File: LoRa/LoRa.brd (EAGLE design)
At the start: 51.7 x 22.8 mm, 27 parts, among them J1 UP2-AH-1-TH, U1 STM32L053C8T6, U2 RFM69HCW, U3 BSS138, U4 BSS138, U5 LM3671MF-3.3/NOPB, X1 uFL/SMA, Y1 ECS-80-S-4X

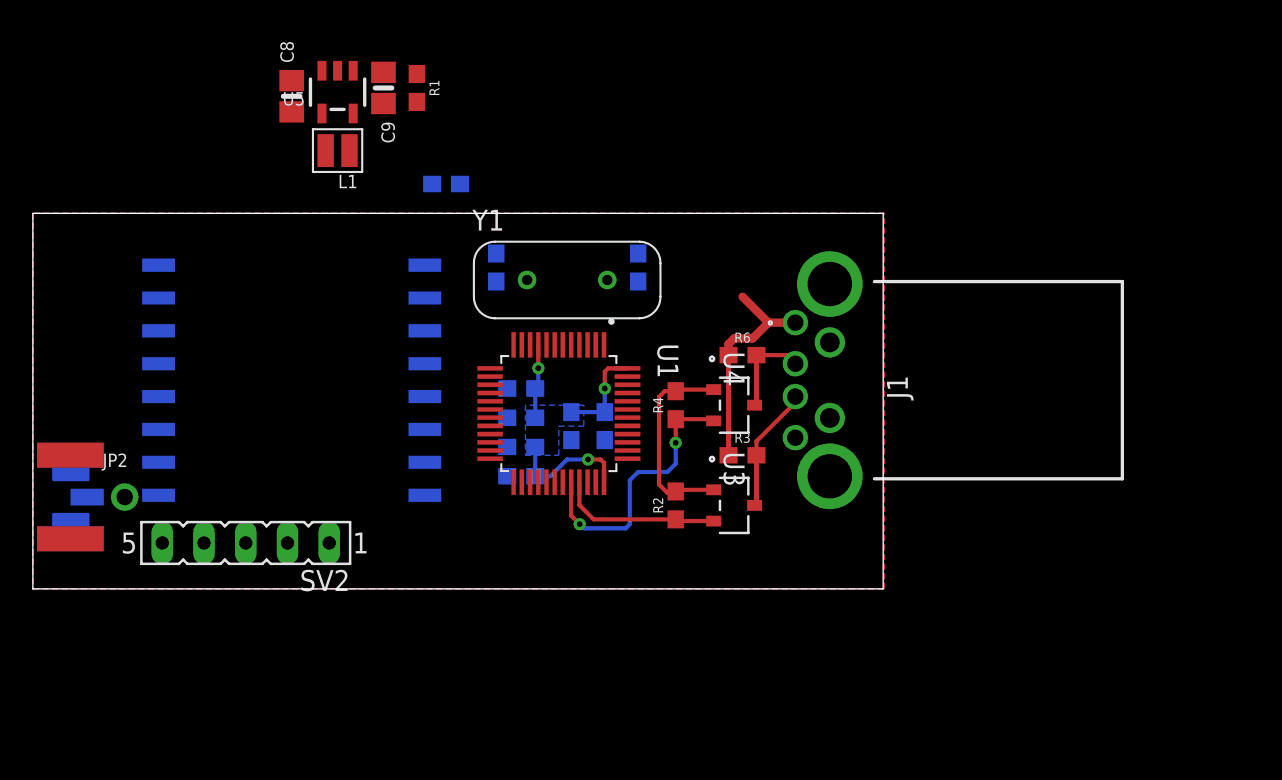
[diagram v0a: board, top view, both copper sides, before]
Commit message: updates
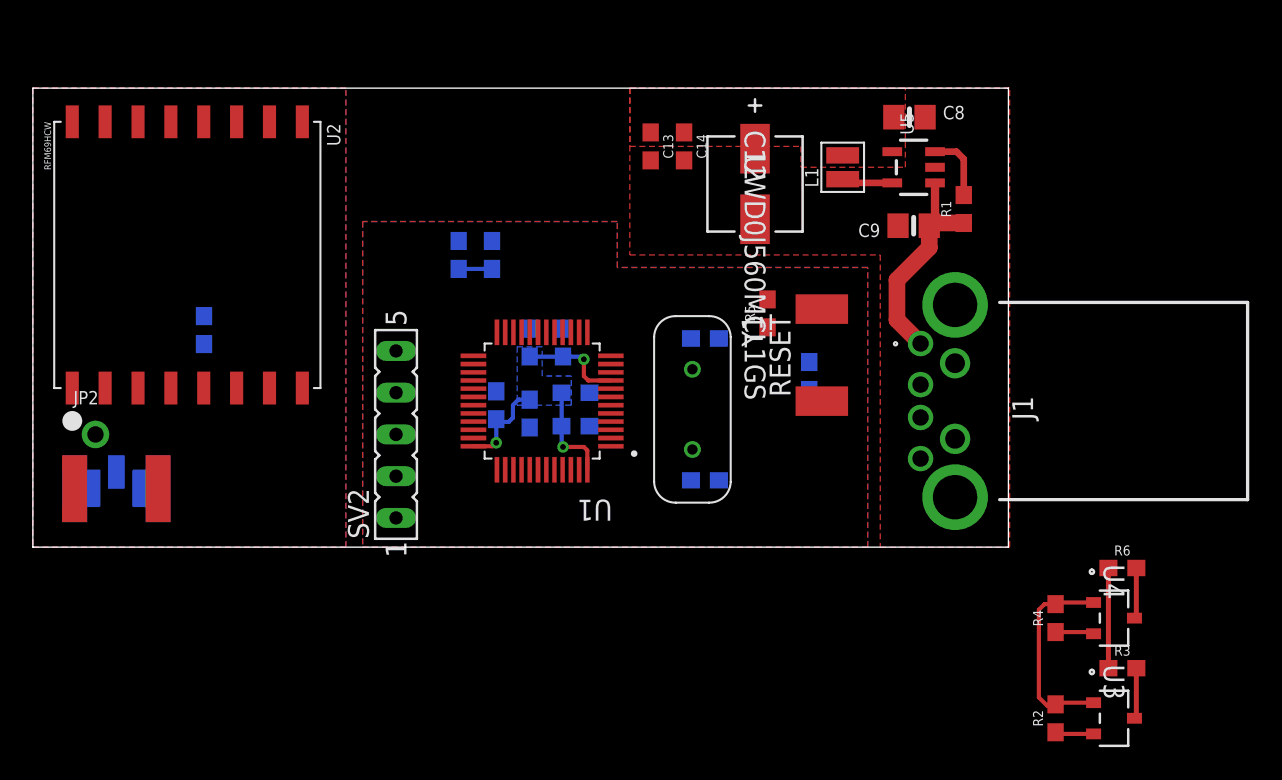
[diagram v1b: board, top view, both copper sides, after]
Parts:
- added C12: UWD0J560MCL1GS, 56uF_Cap_6.3v:PCAP_5X5.8-ELECT
- added C13, C16: 1.0uF, SparkFun-Capacitors:0603
- added C14, C15: 0.1uF, SparkFun-Capacitors:0603
- added C17: 4.7uF, SparkFun-Capacitors:0603
- added R5: 1k, SparkFun-Resistors:0603
- added RESET: (no value), DiscreteComponents:SW_2512
- moved C8 37.6 mm to (53.3, 26.2), turned to 0 degrees
- moved U5 35.3 mm to (53.6, 23.1), turned to 90 degrees
- moved R1 34.1 mm to (56.6, 20.6), turned to 90 degrees
- moved C9 33.3 mm to (53.6, 19.6), turned to 180 degrees
- moved L1 30.8 mm to (49.3, 23.1), turned to 90 degrees
- moved U3 26.5 mm to (65.8, -10.4)
- moved U4 26.5 mm to (65.8, -4.32)
- moved R2 26.5 mm to (62.2, -10.4)
- moved R3 26.5 mm to (66.3, -7.37)
- moved R4 26.5 mm to (62.2, -4.32)
- moved R6 26.5 mm to (66.3, -1.27)
- moved C2 17.2 mm to (10.4, 13.2), turned to 90 degrees
- moved C11 13.6 mm to (40.9, 4.06), turned to 180 degrees
- moved C10 13.4 mm to (40.9, 12.7), turned to 180 degrees
- moved SV2 11.3 mm to (22.1, 6.86), turned to 90 degrees
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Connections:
- new net +3V3: R5.2
- net 3.3V: now also C12.1, C13.1, C14.1, C15.1, C16.1
- net CS: now also U1.14
- net DIO0: now also U1.19
- net GND: now also C12.2, C13.2, C14.2, C15.2, C16.2, C17.2, RESET.1
- net NRST: now also C17.1, R5.1, RESET.2
- net RST: now also U1.18
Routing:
- net USB_DM_3V3: track 17.0 -> 2.35 mm, vias 2 -> 0
- net USB_DP_3V3: track 9.96 -> 2.35 mm
- net 5V: track 13.6 -> 19.9 mm
- net USB_DP_5V: track 7.65 -> 3.09 mm
- net EN: track 0.00 -> 4.13 mm
- net N$2: track 0.00 -> 3.11 mm
- net USB_DM_5V: track 5.68 -> 3.09 mm
- net 3.3V: track 30.6 -> 33.1 mm
- added copper zone on layer 1, net 3.3V
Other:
- board size 51.7 x 22.8 mm -> 59.4 x 27.9 mm
